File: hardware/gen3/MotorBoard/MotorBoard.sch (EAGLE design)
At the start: 265 parts, among them M10O1 TEST_PT, M1O2 TEST_PT, M1O3 TEST_PT, M2O1 TEST_PT, M2O2 TEST_PT, M2O3 TEST_PT, M3O1 TEST_PT, M3O2 TEST_PT, M3O3 TEST_PT, M4O1 TEST_PT, M4O2 TEST_PT, M4O3 TEST_PT, U2 ATMEGA165PV-8AU

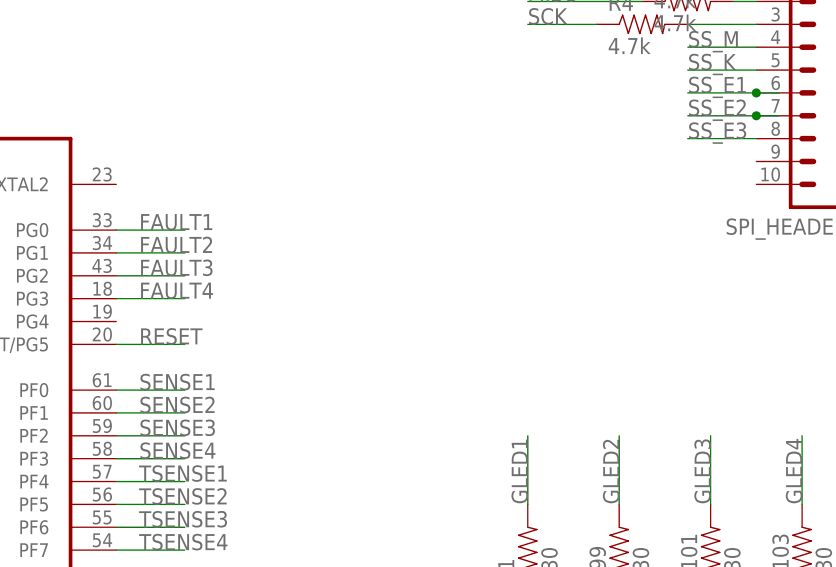
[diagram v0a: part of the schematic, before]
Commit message: motorbrd: just felt like I should commit
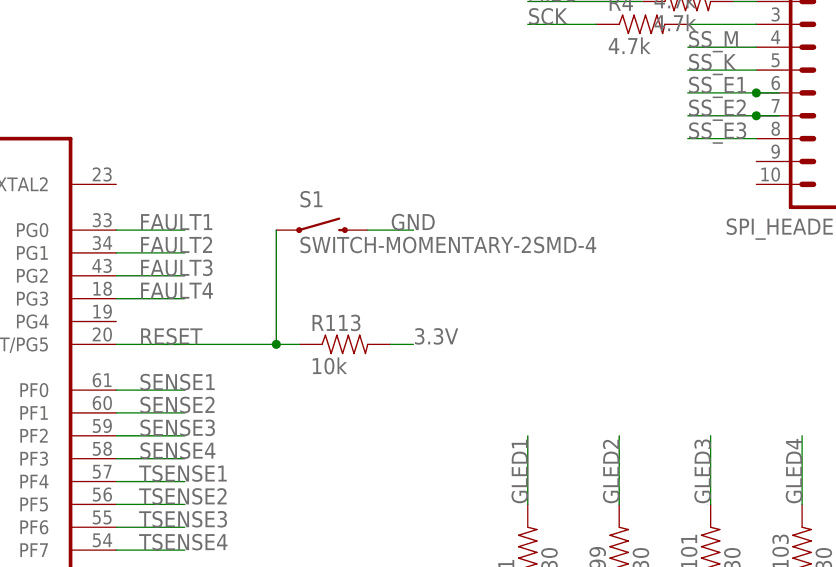
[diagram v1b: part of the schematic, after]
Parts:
- added R113: 10k, SparkFun-Passives:RESISTOR0805-RES
- added S1: SWITCH-MOMENTARY-2SMD-4, SparkFun-Electromechanical:SWITCH-MOMENTARY-2SMD-4
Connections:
- new net RESET1: R113.1, S1.1
- net 3.3V: now also R113.2
- net GND: now also S1.2
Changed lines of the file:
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@@
 <?xml version="1.0" encoding="utf-8"?>
 <!DOCTYPE eagle SYSTEM "eagle.dtd">
-<eagle version="7.2.0">
+<eagle version="6.4">
 <drawing>
 <settings>
@@
 <part name="C57" library="SparkFun-Passives" deviceset="CAP" device="0805" value=".1uF"/>
 <part name="C58" library="SparkFun-Passives" deviceset="CAP" device="0805" value=".1uF"/>
+<part name="S1" library="SparkFun-Electromechanical" deviceset="SWITCH-MOMENTARY-2" device="SMD-4"/>
+<part name="R113" library="SparkFun-Passives" deviceset="RESISTOR" device="0805-RES" value="10k"/>
 </parts>
 <sheets>
@@
 <instance part="C57" gate="G$1" x="327.66" y="223.52"/>
 <instance part="C58" gate="G$1" x="393.7" y="220.98"/>
+<instance part="S1" gate="G$1" x="167.64" y="144.78"/>
+<instance part="R113" gate="G$1" x="170.18" y="132.08"/>
 </instances>
 <busses>
@@
 <label x="485.14" y="152.4" size="1.778" layer="95"/>
 </segment>
+<segment>
+<pinref part="S1" gate="G$1" pin="2"/>
+<wire x1="172.72" y1="144.78" x2="177.8" y2="144.78" width="0.1524" layer="91"/>
+<label x="175.26" y="144.78" size="1.778" layer="95"/>
+</segment>
 </net>
 <net name="3.3V" class="0">
@@
 <label x="469.9" y="165.1" size="1.778" layer="95"/>
 </segment>
+<segment>
+<pinref part="R113" gate="G$1" pin="2"/>
+<wire x1="175.26" y1="132.08" x2="177.8" y2="132.08" width="0.1524" layer="91"/>
+<label x="177.8" y="132.08" size="1.778" layer="95"/>
+</segment>
 </net>
 <net name="MOSI" class="0">
@@
 </segment>
 </net>
+<net name="RESET1" class="0">
+<segment>
+<wire x1="149.86" y1="132.08" x2="162.56" y2="132.08" width="0.1524" layer="91"/>
+<pinref part="S1" gate="G$1" pin="1"/>
+<wire x1="162.56" y1="132.08" x2="162.56" y2="144.78" width="0.1524" layer="91"/>
+<pinref part="R113" gate="G$1" pin="1"/>
+<wire x1="162.56" y1="132.08" x2="165.1" y2="132.08" width="0.1524" layer="91"/>
+<junction x="162.56" y="132.08"/>
+</segment>
+</net>
